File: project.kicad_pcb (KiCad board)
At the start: 2 copper layers, 98.5 x 56 mm, 48 parts, among them J1 Conn_01x04, J2 Conn_01x04, J3 Conn_01x04, J4 Conn_01x04, J5 Conn_01x06, J6 Conn_01x04, J7 Conn_01x04, J9 Conn_02x20_Odd_Even, Q1 BC848, Q2 BC848, Q3 BC848, Q4 BC848, Q5 BC848, Q6 BC848, Q7 BC848, Q8 2N7002, Q9 2N7002

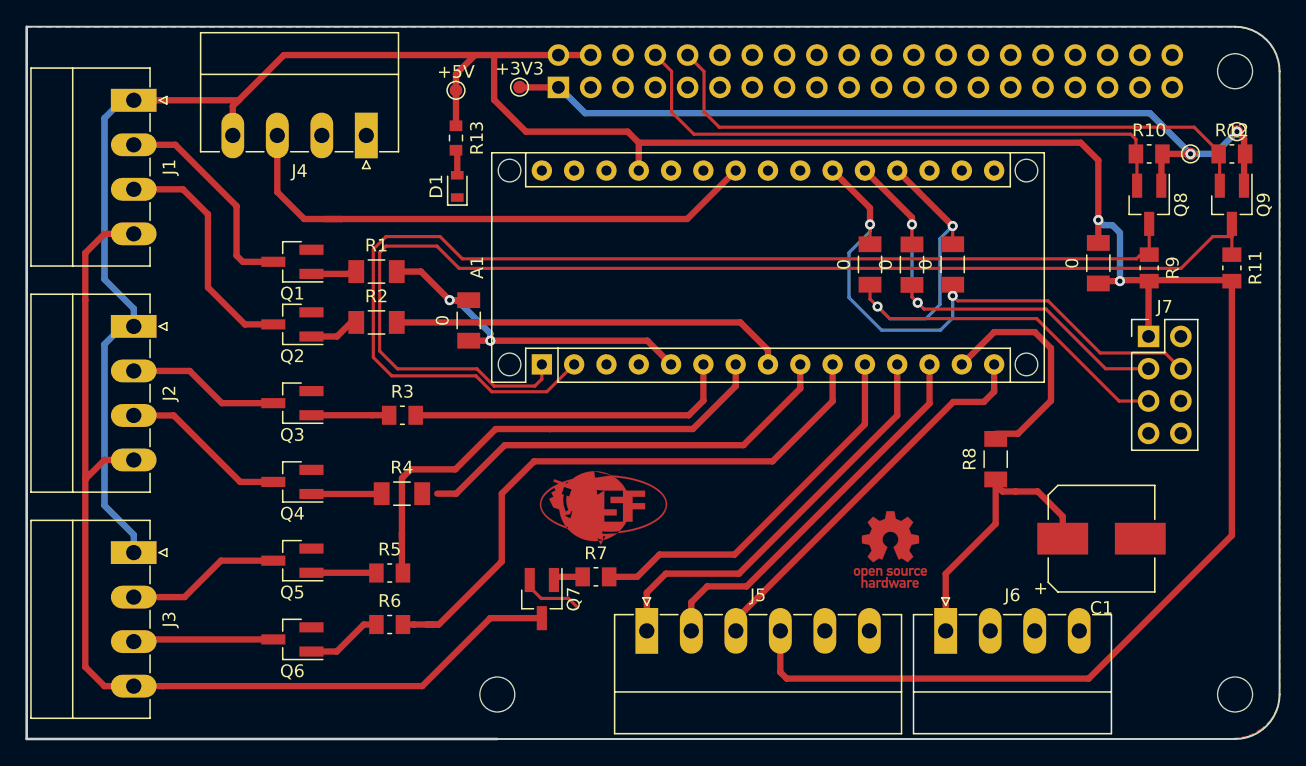
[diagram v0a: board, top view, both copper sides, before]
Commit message: Generated new Gerber files & new Kicad version
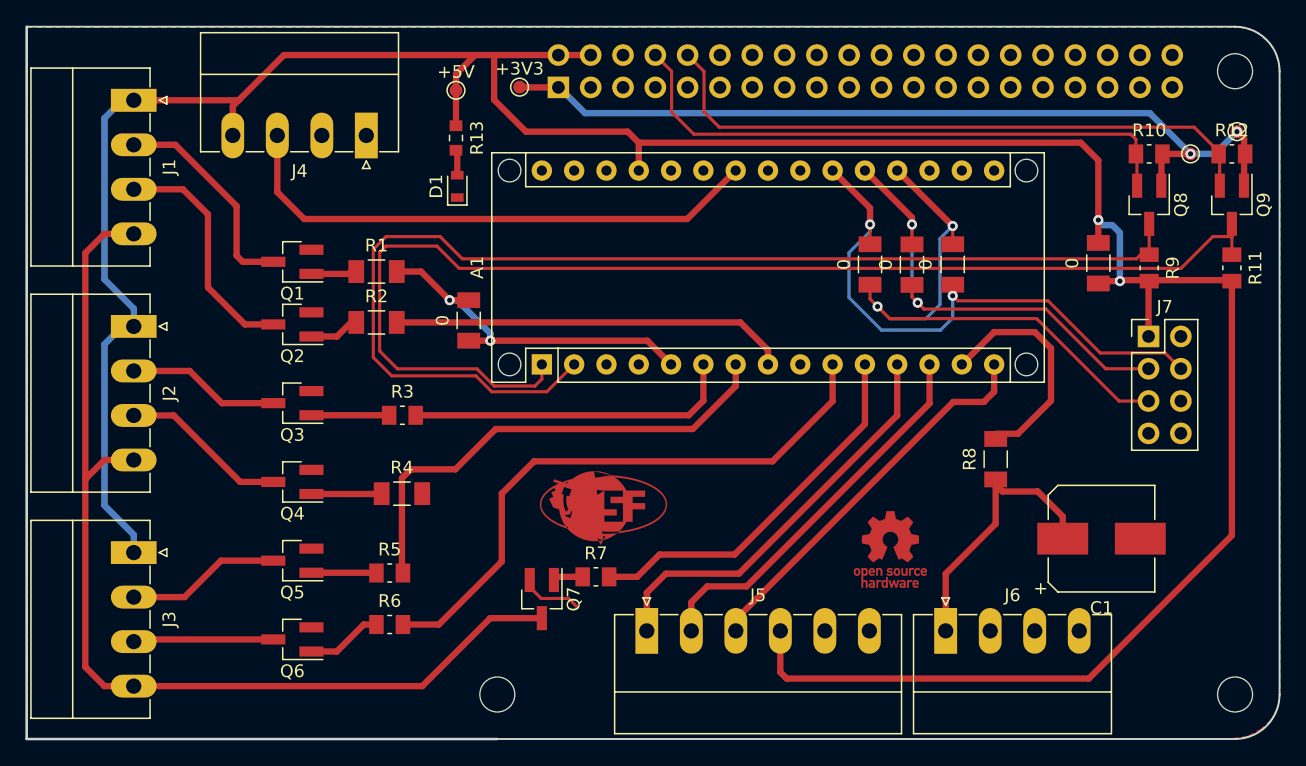
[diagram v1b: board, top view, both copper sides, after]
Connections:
- A1 pad 17: Net-(A1-Pad17) -> unconnected-(A1-3V3-Pad17)
- A1 pad 18: Net-(A1-Pad18) -> unconnected-(A1-AREF-Pad18)
- A1 pad 19: Reset/Abort -> Reset/Abort
- A1 pad 21: CycleStart/Resume -> CycleStart/Resume
- A1 pad 23: Net-(A1-Pad23) -> unconnected-(A1-A4-Pad23)
- A1 pad 25: Net-(A1-Pad25) -> unconnected-(A1-A6-Pad25)
- A1 pad 26: Net-(A1-Pad26) -> unconnected-(A1-A7-Pad26)
- A1 pad 28: Net-(A1-Pad28) -> unconnected-(A1-RESET-Pad28)
- A1 pad 3: Net-(A1-Pad3) -> unconnected-(A1-RESET-Pad3)
- A1 pad 30: Net-(A1-Pad30) -> unconnected-(A1-VIN-Pad30)
- J6 pad 2: Net-(J6-Pad2) -> unconnected-(J6-Pin_2-Pad2)
- J6 pad 3: Net-(J6-Pad3) -> unconnected-(J6-Pin_3-Pad3)
- J7 pad 4: CycleStart/Resume -> CycleStart/Resume
- J7 pad 5: Reset/Abort -> Reset/Abort
- J7 pad 6: Net-(J7-Pad6) -> unconnected-(J7-Pin_6-Pad6)
- J7 pad 7: Net-(J7-Pad7) -> unconnected-(J7-Pin_7-Pad7)
- J7 pad 8: Net-(J7-Pad8) -> unconnected-(J7-Pin_8-Pad8)
- J9 pad 11: Net-(J9-Pad11) -> unconnected-(J9-Pin_11-Pad11)
- J9 pad 12: Net-(J9-Pad12) -> unconnected-(J9-Pin_12-Pad12)
- J9 pad 13: Net-(J9-Pad13) -> unconnected-(J9-Pin_13-Pad13)
- J9 pad 14: Net-(J9-Pad14) -> unconnected-(J9-Pin_14-Pad14)
- J9 pad 15: Net-(J9-Pad15) -> unconnected-(J9-Pin_15-Pad15)
- J9 pad 16: Net-(J9-Pad16) -> unconnected-(J9-Pin_16-Pad16)
- J9 pad 17: Net-(J9-Pad17) -> unconnected-(J9-Pin_17-Pad17)
- J9 pad 18: Net-(J9-Pad18) -> unconnected-(J9-Pin_18-Pad18)
- J9 pad 19: Net-(J9-Pad19) -> unconnected-(J9-Pin_19-Pad19)
- J9 pad 20: Net-(J9-Pad20) -> unconnected-(J9-Pin_20-Pad20)
- J9 pad 21: Net-(J9-Pad21) -> unconnected-(J9-Pin_21-Pad21)
- J9 pad 22: Net-(J9-Pad22) -> unconnected-(J9-Pin_22-Pad22)
- J9 pad 23: Net-(J9-Pad23) -> unconnected-(J9-Pin_23-Pad23)
- J9 pad 24: Net-(J9-Pad24) -> unconnected-(J9-Pin_24-Pad24)
- J9 pad 25: Net-(J9-Pad25) -> unconnected-(J9-Pin_25-Pad25)
- J9 pad 26: Net-(J9-Pad26) -> unconnected-(J9-Pin_26-Pad26)
- J9 pad 29: Net-(J9-Pad29) -> unconnected-(J9-Pin_29-Pad29)
- J9 pad 3: Net-(J9-Pad3) -> unconnected-(J9-Pin_3-Pad3)
- J9 pad 30: Net-(J9-Pad30) -> unconnected-(J9-Pin_30-Pad30)
- J9 pad 31: Net-(J9-Pad31) -> unconnected-(J9-Pin_31-Pad31)
- J9 pad 32: Net-(J9-Pad32) -> unconnected-(J9-Pin_32-Pad32)
- J9 pad 33: Net-(J9-Pad33) -> unconnected-(J9-Pin_33-Pad33)
- J9 pad 34: Net-(J9-Pad34) -> unconnected-(J9-Pin_34-Pad34)
- J9 pad 35: Net-(J9-Pad35) -> unconnected-(J9-Pin_35-Pad35)
- J9 pad 36: Net-(J9-Pad36) -> unconnected-(J9-Pin_36-Pad36)
- J9 pad 37: Net-(J9-Pad37) -> unconnected-(J9-Pin_37-Pad37)
- J9 pad 38: Net-(J9-Pad38) -> unconnected-(J9-Pin_38-Pad38)
- J9 pad 39: Net-(J9-Pad39) -> unconnected-(J9-Pin_39-Pad39)
- J9 pad 40: Net-(J9-Pad40) -> unconnected-(J9-Pin_40-Pad40)
- J9 pad 5: Net-(J9-Pad5) -> unconnected-(J9-Pin_5-Pad5)
- J9 pad 7: Net-(J9-Pad7) -> unconnected-(J9-Pin_7-Pad7)
- J9 pad 9: Net-(J9-Pad9) -> unconnected-(J9-Pin_9-Pad9)
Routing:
- net DirY: track 33.9 -> 0.00 mm
- net +5V: track 235.3 -> 233.5 mm
- net TX_5V: track 95.8 -> 94.3 mm
- net Probe: track 44.3 -> 42.9 mm
- net DirZOut: track 11.9 -> 11.0 mm
- net DirZ: track 47.7 -> 47.2 mm
- net StepZ: track 38.9 -> 38.4 mm
- net (no net): vias 3 -> 0
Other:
- net class Default removed
- net class GND removed
- net class komm removed
